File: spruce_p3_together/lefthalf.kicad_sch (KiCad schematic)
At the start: 22 parts, among them J1 USB_C_Receptacle_USB2.0, U1 STM32F072CBT6, U2 PRTR5V0U2X, U7 TRRS

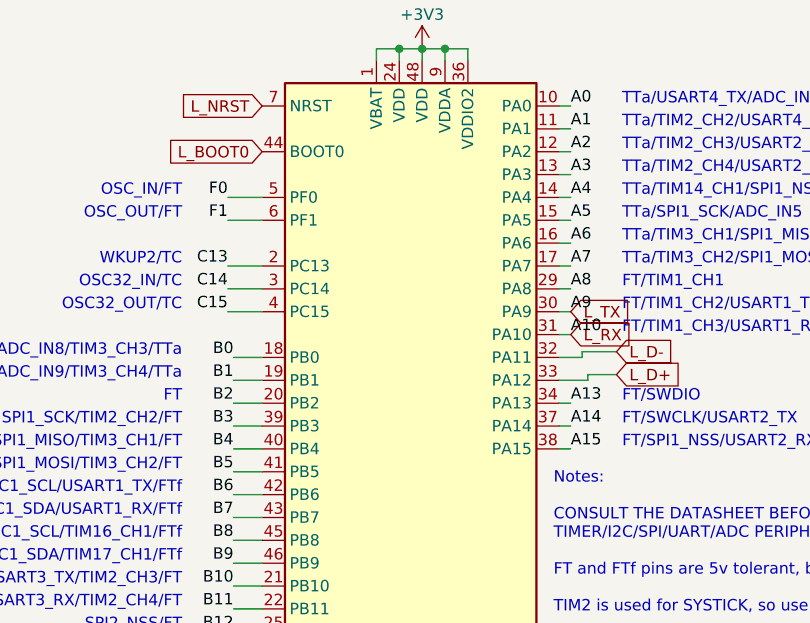
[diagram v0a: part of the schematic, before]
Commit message: routing for keys
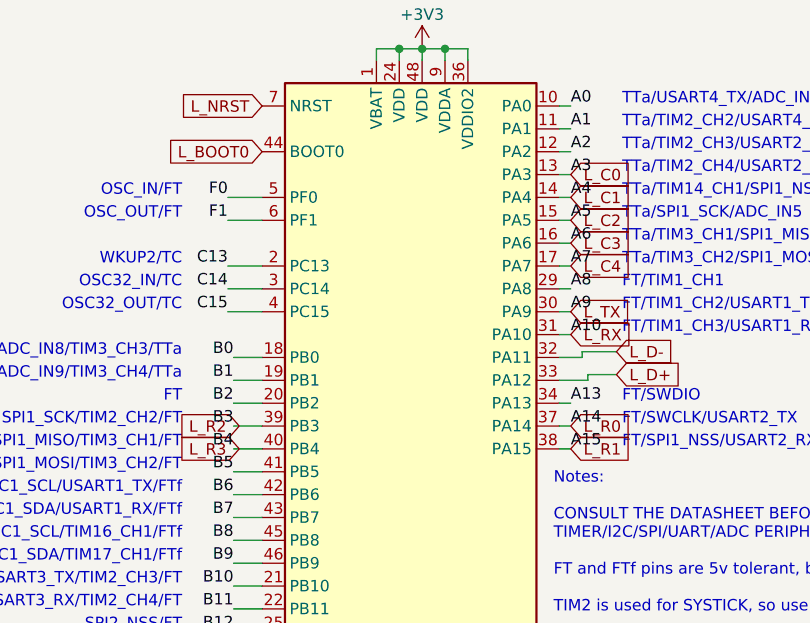
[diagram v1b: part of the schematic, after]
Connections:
- net A14 renamed L_R0
- net A15 renamed L_R1
- net A3 renamed L_C0
- net A4 renamed L_C1
- net A5 renamed L_C2
- net A6 renamed L_C3
- net A7 renamed L_C4
- net B3 renamed L_R2
- net B4 renamed L_R3
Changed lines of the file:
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@@
+    )
+  )
+  (global_label "L_R1" (shape input) (at 96.52 66.04 0) (fields_autoplaced)
+    (effects (font (size 1.27 1.27)) (justify left))
+    (property "Intersheetrefs" "${INTERSHEET_REFS}" (at 103.9804 66.04 0)
+      (effects (font (size 1.27 1.27)) (justify left) hide)
+    )
+  )
+  (global_label "L_C0" (shape input) (at 96.52 35.56 0) (fields_autoplaced)
+    (effects (font (size 1.27 1.27)) (justify left))
+    (property "Intersheetrefs" "${INTERSHEET_REFS}" (at 103.9804 35.56 0)
+      (effects (font (size 1.27 1.27)) (justify left) hide)
     )
   )
@@
     )
   )
+  (global_label "L_R0" (shape input) (at 96.52 63.5 0) (fields_autoplaced)
+    (effects (font (size 1.27 1.27)) (justify left))
+    (property "Intersheetrefs" "${INTERSHEET_REFS}" (at 103.9804 63.5 0)
+      (effects (font (size 1.27 1.27)) (justify left) hide)
+    )
+  )
+  (global_label "L_C1" (shape input) (at 96.52 38.1 0) (fields_autoplaced)
+    (effects (font (size 1.27 1.27)) (justify left))
+    (property "Intersheetrefs" "${INTERSHEET_REFS}" (at 103.9804 38.1 0)
+      (effects (font (size 1.27 1.27)) (justify left) hide)
+    )
+  )
   (global_label "L_TX" (shape input) (at 96.52 50.8 0) (fields_autoplaced)
     (effects (font (size 1.27 1.27)) (justify left))
@@
     (effects (font (size 1.27 1.27)) (justify right))
     (property "Intersheetrefs" "${INTERSHEET_REFS}" (at 51.141 33.02 0)
+      (effects (font (size 1.27 1.27)) (justify right) hide)
+    )
+  )
+  (global_label "L_R2" (shape input) (at 59.69 63.5 180) (fields_autoplaced)
+    (effects (font (size 1.27 1.27)) (justify right))
+    (property "Intersheetrefs" "${INTERSHEET_REFS}" (at 52.2296 63.5 0)
       (effects (font (size 1.27 1.27)) (justify right) hide)
     )
@@
     )
   )
+  (global_label "L_R3" (shape input) (at 59.69 66.04 180) (fields_autoplaced)
+    (effects (font (size 1.27 1.27)) (justify right))
+    (property "Intersheetrefs" "${INTERSHEET_REFS}" (at 52.2296 66.04 0)
+      (effects (font (size 1.27 1.27)) (justify right) hide)
+    )
+  )
+  (global_label "L_C4" (shape input) (at 96.52 45.72 0) (fields_autoplaced)
+    (effects (font (size 1.27 1.27)) (justify left))
+    (property "Intersheetrefs" "${INTERSHEET_REFS}" (at 103.9804 45.72 0)
+      (effects (font (size 1.27 1.27)) (justify left) hide)
+    )
+  )
   (global_label "L_VBUS" (shape input) (at 67.945 154.305 180) (fields_autoplaced)
     (effects (font (size 1.27 1.27)) (justify right))
@@
       (effects (font (size 1.27 1.27)) (justify left) hide)
     )
+  )
+  (global_label "L_C3" (shape input) (at 96.52 43.18 0) (fields_autoplaced)
+    (effects (font (size 1.27 1.27)) (justify left))
+    (property "Intersheetrefs" "${INTERSHEET_REFS}" (at 103.9804 43.18 0)
+      (effects (font (size 1.27 1.27)) (justify left) hide)
+    )
+  )
+  (global_label "L_C2" (shape input) (at 96.52 40.64 0) (fields_autoplaced)
+    (effects (font (size 1.27 1.27)) (justify left))
+    (property "Intersheetrefs" "${INTERSHEET_REFS}" (at 103.9804 40.64 0)
+      (effects (font (size 1.27 1.27)) (justify left) hide)
+    )
